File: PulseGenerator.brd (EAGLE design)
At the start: 60.6 x 30 mm, 22 parts, among them IC1 MC34063AD, T1 2N2369, X1 1-227161-0

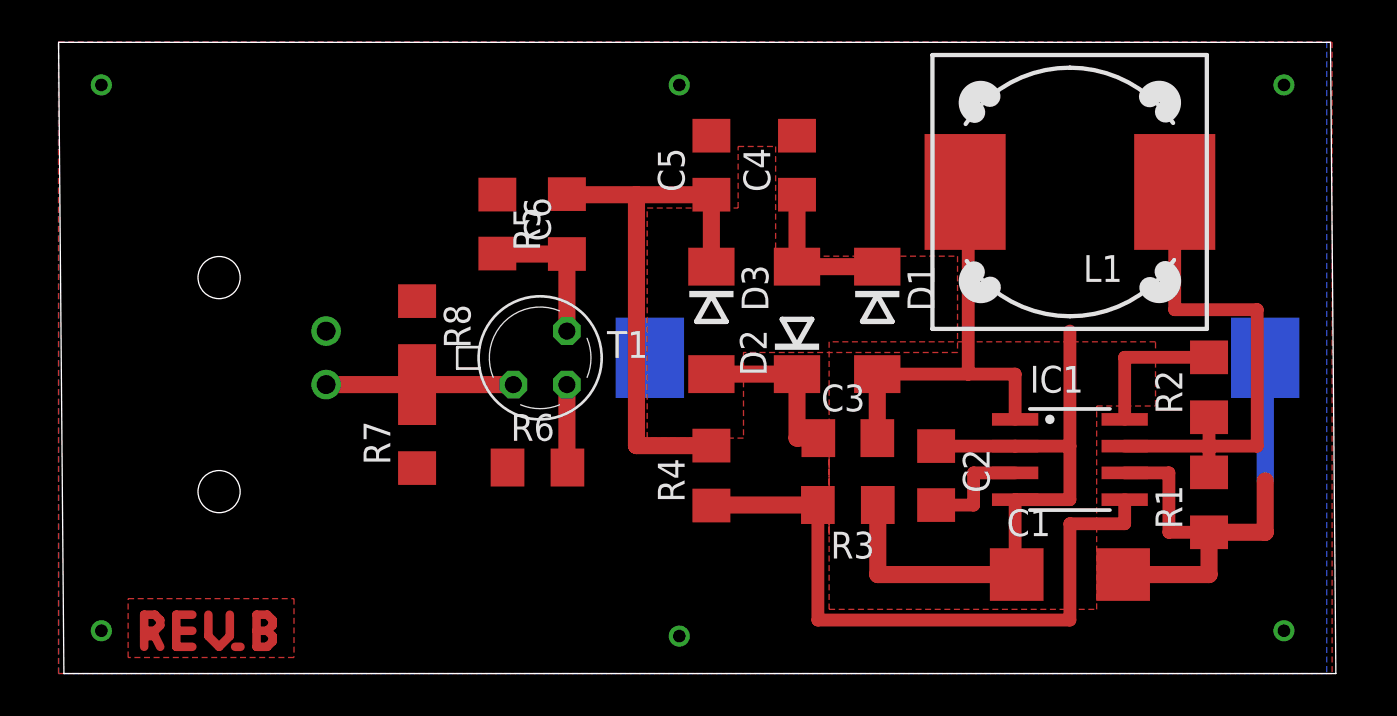
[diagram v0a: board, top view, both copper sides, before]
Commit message: Commit of the current version
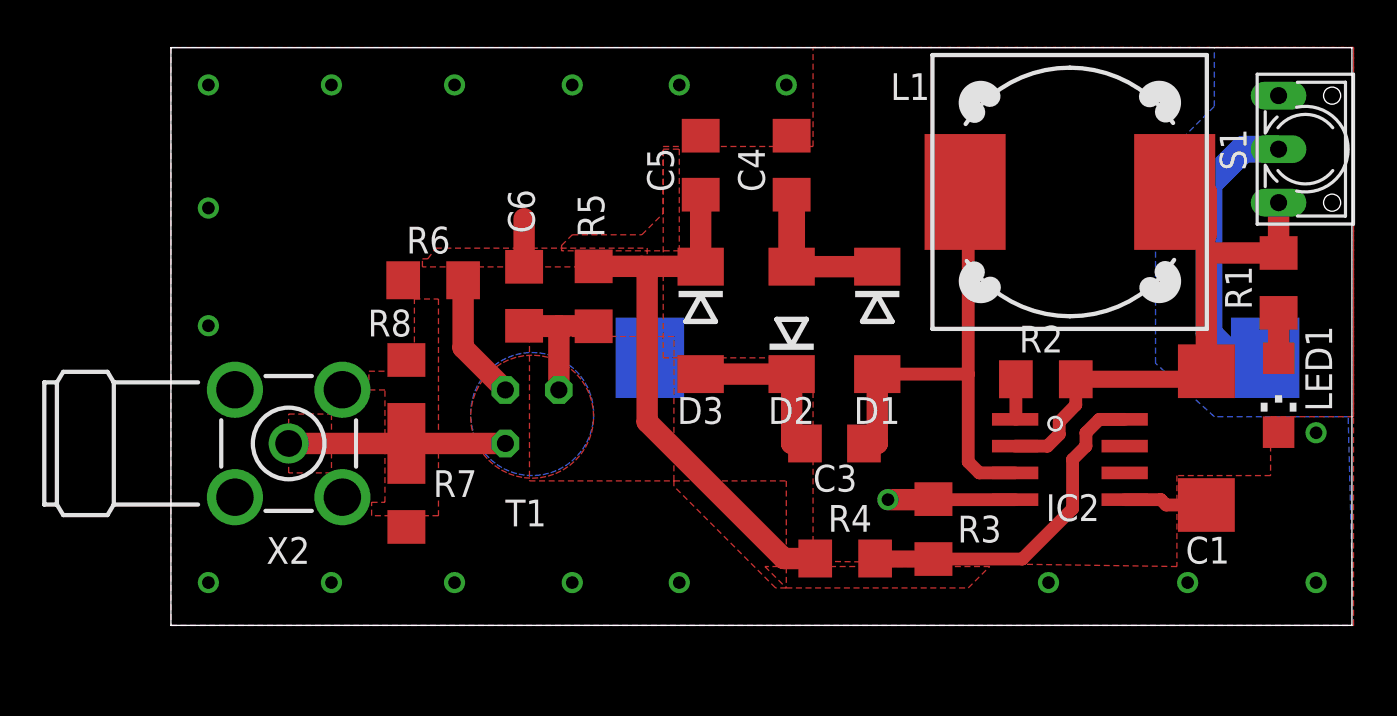
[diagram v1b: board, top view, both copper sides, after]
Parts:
- removed C2: 220pF, rcl:C1206
- removed IC1: MC34063AD, v-reg-3:SO08
- removed X1: 1-227161-0, con-coax:AMP_227161
- added GOLD_ORB_SM1: OSHWLOGO_GOLD_ORB_SM, bfl:OSHW2
- added IC2: LT1073-SO08, lt1073:SO08
- added LED1: (no value), led:CHIPLED_1206
- added S1: 9450-1, switch-misc:9450-1
- added X2: (no value), con-coax:BU-SMA-H
- C1: device rcl:C/6032-28R -> rcl:D/7343-31R
- L1: value DR125 -> 150uH
- R1: value 0.76 -> 220
- moved R1 10.9 mm to (57.7, 37.6)
- moved R6 10.2 mm to (17.5, 37.7)
- moved C1 9.16 mm to (54.2, 30.2), turned to 90 degrees
- moved R2 7.76 mm to (46.6, 33.0), turned to 0 degrees
- moved R4 7.47 mm to (37.1, 24.5), turned to 180 degrees
- moved R3 4.22 mm to (41.3, 25.9), turned to 270 degrees
- moved C6 3.66 mm to (21.8, 37.0)
- moved R5 3.66 mm to (25.1, 37.0)
- moved R7 2.84 mm to (16.3, 27.4)
- moved R8 2.84 mm to (16.3, 32.5)
- moved T1 2.82 mm to (22.2, 31.2), flipped to the bottom, turned to 90 degrees
- moved C3 0.68 mm to (36.6, 30.0)
- moved C5 0.51 mm to (30.2, 43.2)
- moved D3 0.51 mm to (30.2, 35.8)
- moved C4 0.25 mm to (34.5, 43.2)
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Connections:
- net GND: now also IC2.4, IC2.5, LED1.C, X2.2, X2.3, X2.4, X2.5; no longer C2.1, IC1.2, IC1.4, X1.2
- net N$11: now also X2.1; no longer X1.1
- net N$2: now also LED1.A, R1.1; no longer IC1.8, R2.2
- net N$3: now also G1.+, S1.2; no longer IC1.7, L1.1, R1.2, R2.1
- net N$5: now also IC2.1, R2.1; no longer C2.2, IC1.3
- net N$8: now also IC2.3; no longer IC1.1
- net N$9: now also IC2.8; no longer IC1.5
- net VCC: now also IC2.2, L1.1, R1.2, R2.2, S1.3; no longer G1.+, IC1.6, R1.1
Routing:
- net GND: track 31.2 -> 13.1 mm, vias 6 -> 18
- net N$9: track 30.8 -> 16.5 mm
- net N$3: track 24.9 -> 14.3 mm
- net N$25: track 4.99 -> 0.00 mm
- net N$2: track 6.95 -> 2.16 mm
- net N$17: track 4.59 -> 0.00 mm
- net VCC: track 24.0 -> 27.8 mm
- net N$21: track 3.81 -> 0.00 mm
- net N$23: track 3.47 -> 0.00 mm
- net N$5: track 5.28 -> 1.94 mm
- net N$8: track 20.8 -> 23.8 mm
- net N$10: track 3.96 -> 6.04 mm
- net N$11: track 11.1 -> 12.5 mm
- net N$7: track 25.8 -> 26.7 mm
- net N$6: track 6.98 -> 6.36 mm
- added copper zone on layer 16, net N$12
- added copper zone on layer 1, net N$14
- added copper zone on layer 1, net N$15
- added copper zone on layer 1, net N$26
- added copper zone on layer 1, net N$27
- added copper zone on layer 1, net N$28
- added copper zone on layer 1, net N$29
- added copper zone on layer 1, net N$30
- added copper zone on layer 1, net N$31
- removed copper zone on layer 1, net N$12
- removed copper zone on layer 1, net N$16
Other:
- board size 60.6 x 30 mm -> 56.1 x 27.4 mm
- board text added: "PulseGen"
- board text added: "Rev.C"
